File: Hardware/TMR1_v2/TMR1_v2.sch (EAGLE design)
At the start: 47 parts, among them U1 ATMEGA328P_TQFP, U2 MCP79410I/SN, Y1 32.768kHz

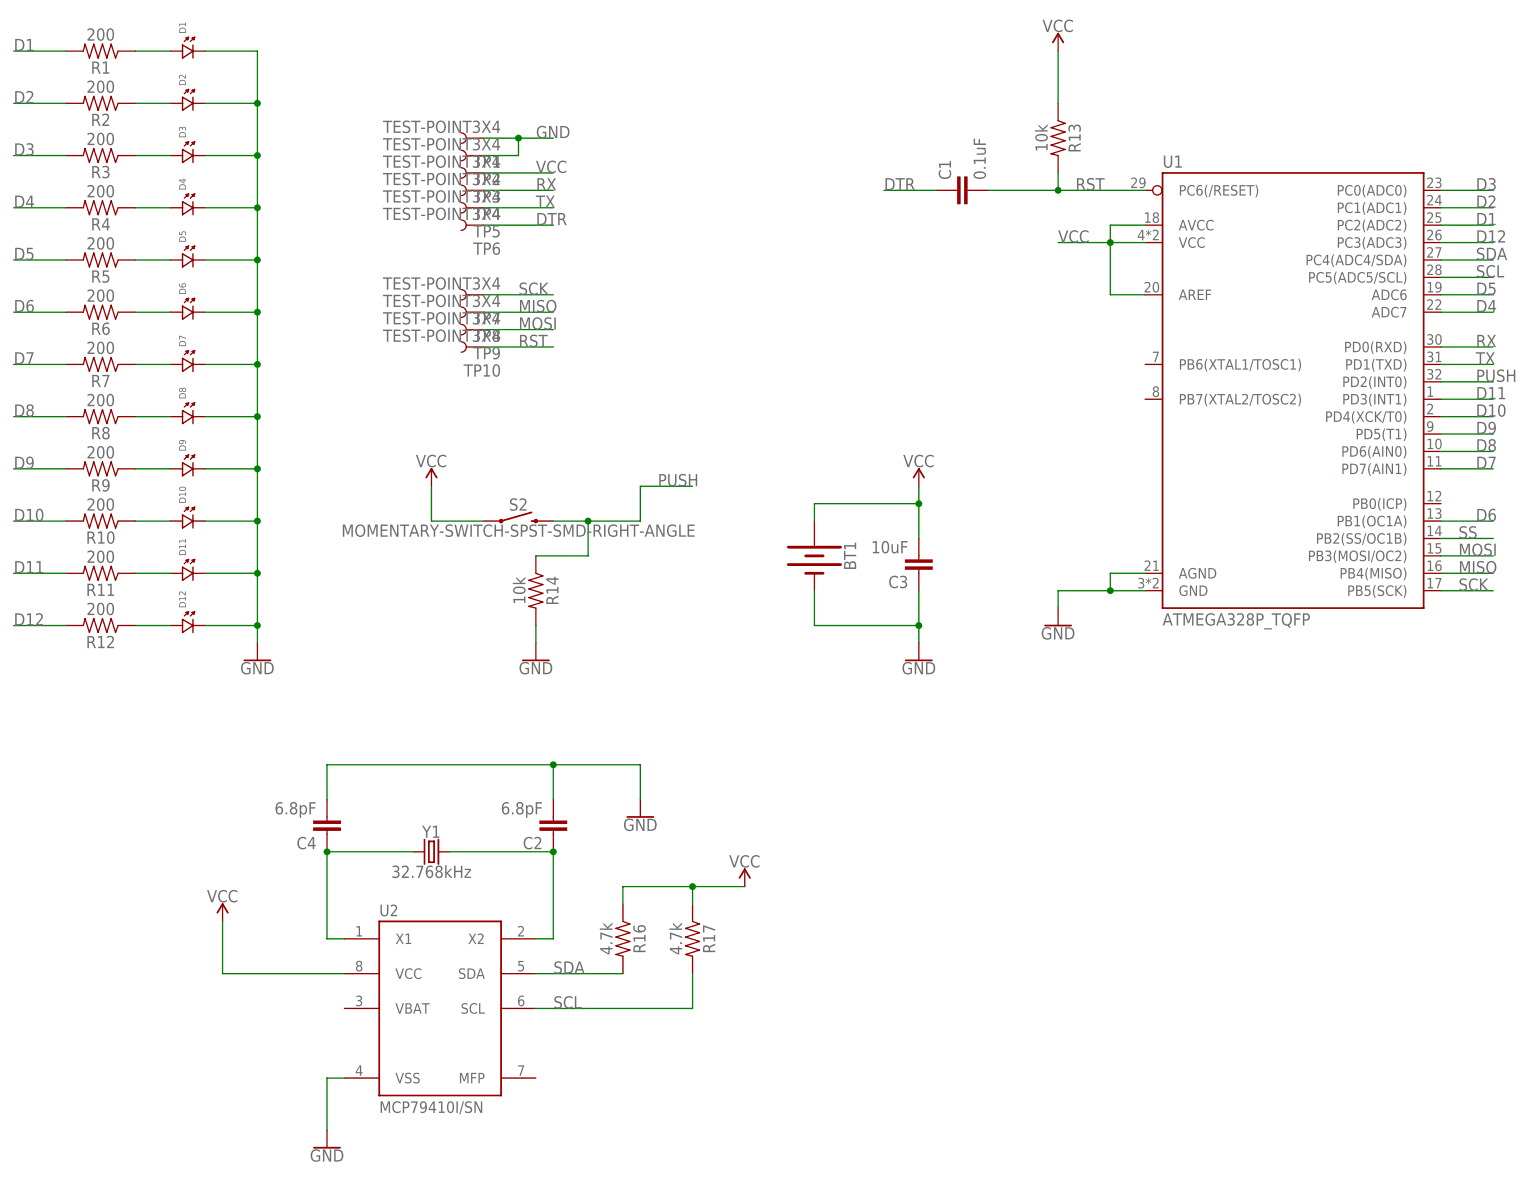
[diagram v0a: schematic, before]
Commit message: std easy schematic with all elements in board before route
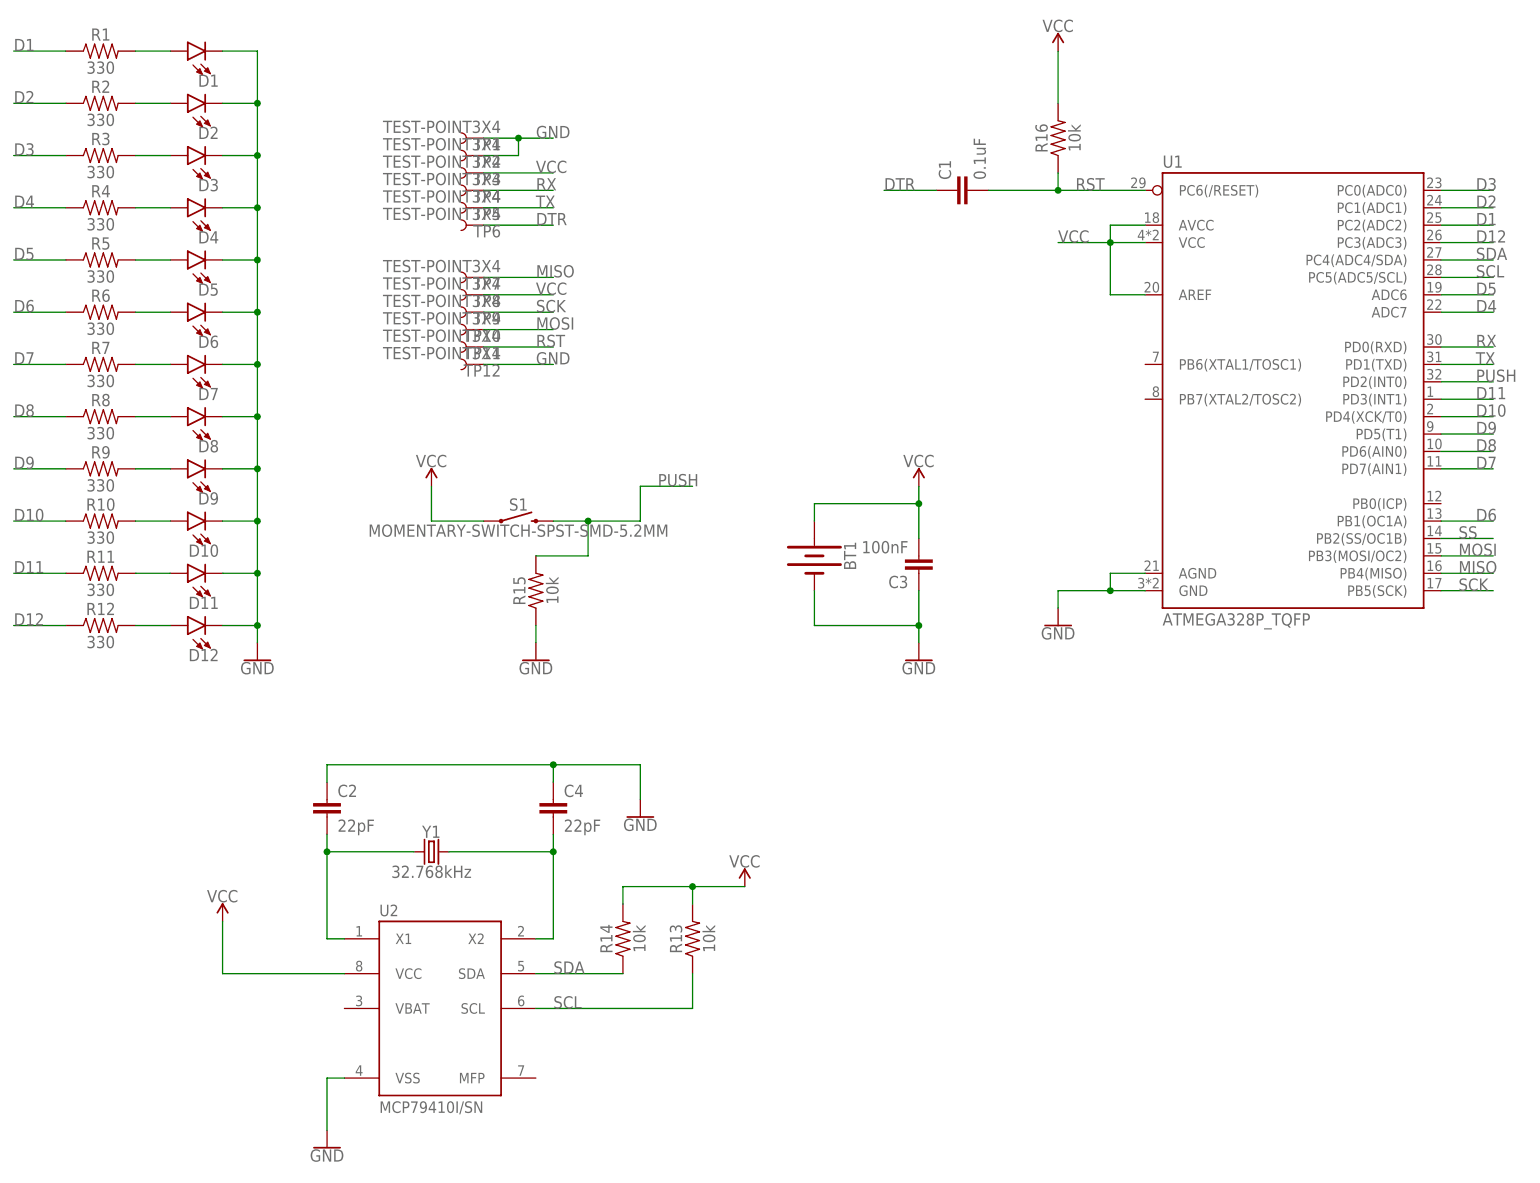
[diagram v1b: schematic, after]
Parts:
- removed R17: 4.7k, SparkFun-Resistors:RESISTOR0402
- removed S2: MOMENTARY-SWITCH-SPST-SMD-RIGHT-ANGLE, SparkFun-Switches:MOMENTARY-SWITCH-SPST-SMD-RIGHT-ANGLE
- added R15: 10k, SparkFun-Resistors:10KOHM-0603-1/10W-1%
- added S1: MOMENTARY-SWITCH-SPST-SMD-5.2MM, SparkFun-Switches:MOMENTARY-SWITCH-SPST-SMD-5.2MM
- added TP11, TP12: TEST-POINT3X4, SparkFun-Connectors:TEST-POINT3X4
- C2, C4: value 6.8pF -> 22pF; device SparkFun-Capacitors:0.1UF-0402-16V-10% -> SparkFun-Capacitors:22PF-0603-50V-5%
- C3: value 10uF -> 100nF
- D1, D10, D11, D12, D2, D3, D4, D5, D6, D7, D8, D9: device standardparts:LED.0402 -> SparkFun-LED:LED0603
- R1, R10, R11, R12, R2, R3, R4, R5, R6, R7, R8, R9: value 200 -> 330; device SparkFun-Resistors:RESISTOR0402 -> SparkFun-Resistors:330OHM-0603-1/10W-1%
- R13, R14: device SparkFun-Resistors:RESISTOR0402 -> SparkFun-Resistors:10KOHM-0603-1/10W-1%
- R16: value 4.7k -> 10k; device SparkFun-Resistors:RESISTOR0402 -> SparkFun-Resistors:10KOHM-0603-1/10W-1%
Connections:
- net D1: now also R1.1; no longer R1.2
- net D10: now also R10.1; no longer R10.2
- net D11: now also R11.1; no longer R11.2
- net D12: now also R12.1; no longer R12.2
- net D2: now also R2.1; no longer R2.2
- net D3: now also R3.1; no longer R3.2
- net D4: now also R4.1; no longer R4.2
- net D5: now also R5.1; no longer R5.2
- net D6: now also R6.1; no longer R6.2
- net D7: now also R7.1; no longer R7.2
- net D8: now also R8.1; no longer R8.2
- net D9: now also R9.1; no longer R9.2
- net GND: now also C2.1, C4.1, D1.C, D10.C, D11.C, D12.C, D2.C, D3.C, D4.C, D5.C, D6.C, D7.C, D8.C, D9.C, R15.1, TP12.1; no longer C2.2, C4.2, D1.2, D10.2, D11.2, D12.2, D2.2, D3.2, D4.2, D5.2, D6.2, D7.2, D8.2, D9.2, R14.2
- net MISO: now also TP7.1; no longer TP8.1
- net MOSI: now also TP10.1; no longer TP9.1
- net N$1: now also D8.A, R8.2; no longer D8.1, R8.1
- net N$10: now also C4.2; no longer C2.1
- net N$18: now also D9.A, R9.2; no longer D9.1, R9.1
- net N$2: now also D7.A, R7.2; no longer D7.1, R7.1
- net N$20: now also D10.A, R10.2; no longer D10.1, R10.1
- net N$22: now also D11.A, R11.2; no longer D11.1, R11.1
- net N$24: now also D12.A, R12.2; no longer D12.1, R12.1
- net N$3: now also D6.A, R6.2; no longer D6.1, R6.1
- net N$4: now also D5.A, R5.2; no longer D5.1, R5.1
- net N$5: now also D4.A, R4.2; no longer D4.1, R4.1
- net N$6: now also D3.A, R3.2; no longer D3.1, R3.1
- net N$7: now also D2.A, R2.2; no longer D2.1, R2.1
- net N$8: now also D1.A, R1.2; no longer D1.1, R1.1
- net N$9: now also C2.2; no longer C4.1
- net PUSH: now also R15.2, S1.2; no longer R14.1, S2.2
- net RST: now also R16.1, TP11.1; no longer R13.2, TP10.1
- net SCK: now also TP9.1; no longer TP7.1
- net SCL: now also R13.1; no longer R17.2
- net SDA: now also R14.1; no longer R16.2
- net VCC: now also R13.2, R14.2, R16.2, S1.1, TP8.1; no longer R13.1, R16.1, R17.1, S2.1
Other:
- moved on the sheet: C2, C4, R1, R10, R11, R12, R13, R14, R16, R2, R3, R4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
